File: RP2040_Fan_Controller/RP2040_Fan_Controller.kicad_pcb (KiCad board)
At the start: 2 copper layers, 52 x 80 mm, 29 parts, among them J1 USB

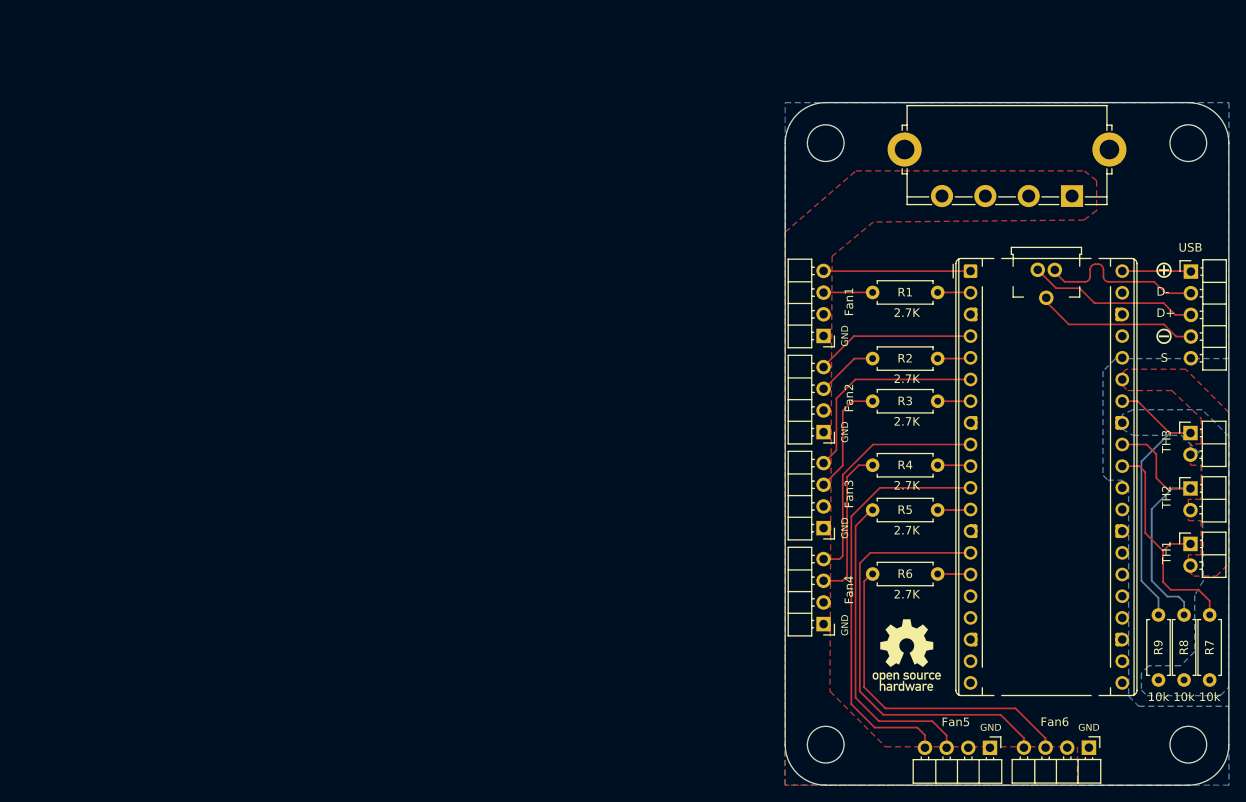
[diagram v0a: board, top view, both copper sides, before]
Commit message: PCB-Rev 1.0.0
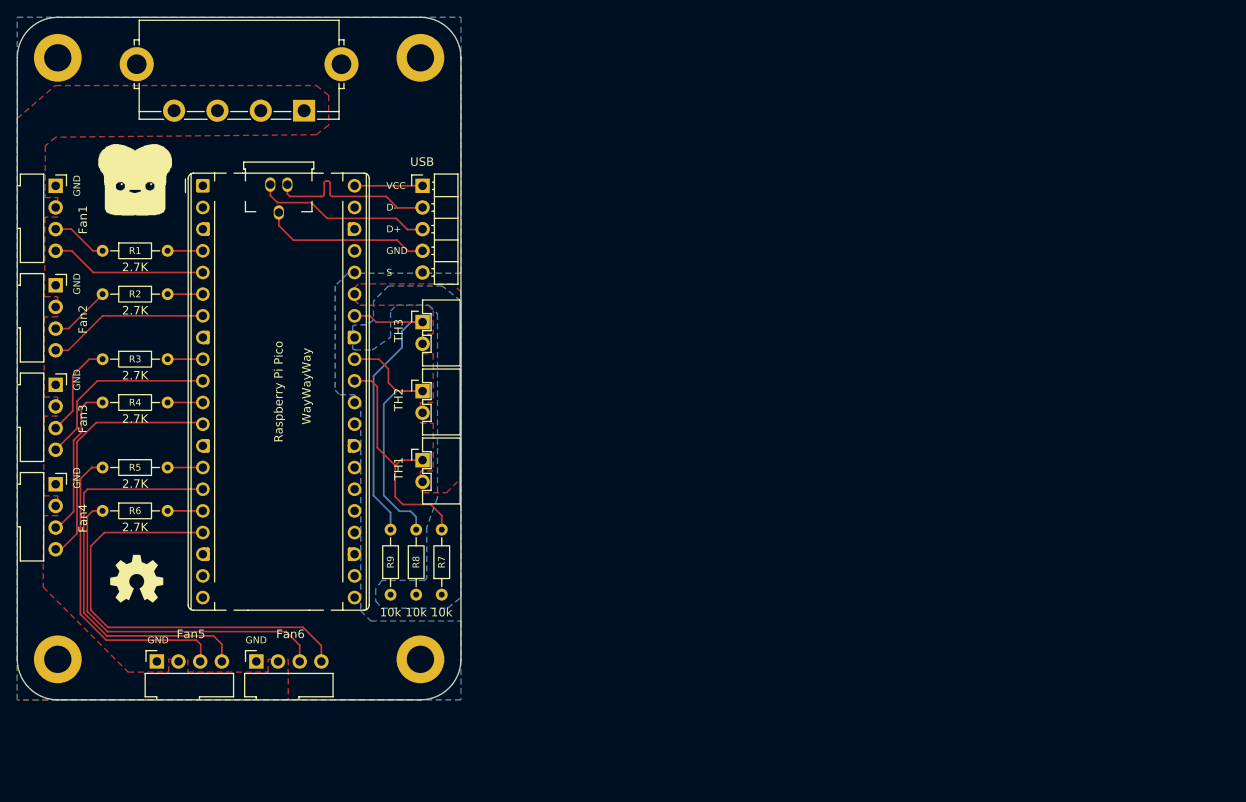
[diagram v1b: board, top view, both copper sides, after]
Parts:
- added G***: Toast_Invert, Library:Toast_Invert, F.Cu at (73.8, 59.2)
- R1, R2, R3, R4, R5, R6, R7, R8, R9: footprint Resistor_THT:R_Axial_DIN0207_L6.3mm_D2.5mm_P7.62mm_Horizontal -> Resistor_THT:R_Axial_DIN0204_L3.6mm_D1.6mm_P7.62mm_Horizontal
- REF** (x3): value MountingHole_4.3mm_M4 -> MountingHole_3.2mm_M3_DIN965_Pad; footprint MountingHole:MountingHole_4.3mm_M4 -> MountingHole:MountingHole_3.2mm_M3_DIN965_Pad
- REF**: value MountingHole_4.3mm_M4 -> (none); footprint MountingHole:MountingHole_4.3mm_M4 -> MountingHole:MountingHole_3.2mm_M3_DIN965_Pad
- moved Fan1 100.4 mm to (55.7, 59.8), turned to 0 degrees
- moved Fan2 100.3 mm to (55.7, 71.4), turned to 0 degrees
- moved Fan3 100.2 mm to (55.7, 83.1), turned to 0 degrees
- moved Fan4 100.2 mm to (55.7, 94.7), turned to 0 degrees
- moved Fan5 97.6 mm to (76.4, 124.3), turned to 90 degrees
- moved Fan6 97.6 mm to (88.0, 124.3), turned to 90 degrees
- moved TH3 90.9 mm to (107.5, 75.7)
- moved TH2 90.7 mm to (107.5, 83.8)
- moved J1 90.6 mm to (107.5, 59.8)
- moved R2 90.6 mm to (70.0, 72.5)
- moved R7 90.6 mm to (109.8, 107.7)
- moved R8 90.6 mm to (106.8, 107.7)
- moved R9 90.6 mm to (103.8, 107.7)
- moved REF** 90.6 mm to (64.8, 44.8)
- moved REF** 90.6 mm to (93.6, 51.0)
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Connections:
- A1 pad 1: PWM_FAN1 -> unconnected-(A1-GPIO0-Pad1)
- A1 pad 10: RPM_FAN4 -> PWM_FAN3
- A1 pad 11: PWM_FAN5 -> RPM_FAN4
- A1 pad 12: RPM_FAN5 -> PWM_FAN4
- A1 pad 14: PWM_FAN6 -> RPM_FAN5
- A1 pad 15: RPM_FAN6 -> PWM_FAN5
- A1 pad 16: unconnected-(A1-GPIO12-Pad16) -> RPM_FAN6
- A1 pad 17: unconnected-(A1-GPIO13-Pad17) -> PWM_FAN6
- A1 pad 2: RPM_FAN1 -> unconnected-(A1-GPIO1-Pad2)
- A1 pad 4: PWM_FAN2 -> RPM_FAN1
- A1 pad 5: RPM_FAN2 -> PWM_FAN1
- A1 pad 6: PWM_FAN3 -> RPM_FAN2
- A1 pad 7: RPM_FAN3 -> PWM_FAN2
- A1 pad 9: PWM_FAN4 -> RPM_FAN3
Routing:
- net Net-(Fan6-Tacho): track 37.7 -> 41.5 mm
- net Net-(Fan3-Tacho): track 14.3 -> 10.6 mm
- net PWM_FAN3: track 25.2 -> 21.7 mm
- net Net-(Fan4-Tacho): track 19.0 -> 17.6 mm
- net PWM_FAN6: track 50.5 -> 51.8 mm
- net ADC_2: track 35.4 -> 36.5 mm
- net Net-(Fan2-Tacho): track 7.90 -> 6.95 mm
- net USB_GND: track 18.8 -> 19.7 mm
- net Net-(Fan1-Tacho): track 5.70 -> 6.55 mm
- net PWM_FAN5: track 48.5 -> 47.8 mm
- net USB_DM: track 20.1 -> 20.8 mm
- net PWM_FAN1: track 17.6 -> 18.3 mm
- net PWM_FAN2: track 19.3 -> 18.7 mm
- net ADC_1: track 31.8 -> 32.5 mm
- net USB_DP: track 20.2 -> 20.8 mm
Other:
- board text added: "VCC"
- board text added: "WayWayWay"
- board text added: "https://github.com/mietzen/RP-Pico-Fan-Controller"
- board text removed: "https://github.com/mietzen/RP2040-Fan-Controller"
- board text removed: "⊕"
- board text removed: "⊖"
